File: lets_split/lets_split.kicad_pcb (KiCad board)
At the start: 2 copper layers, 112 x 79 mm, 62 parts, among them J1 3PIN, J2 6PIN, J3 3PIN, SW1 SW_PUSH, SW10 SW_PUSH, SW11 SW_PUSH, SW12 SW_PUSH, SW13 SW_PUSH, SW14 SW_PUSH, SW15 SW_PUSH, SW16 SW_PUSH, SW17 SW_PUSH, SW18 SW_PUSH, SW19 SW_PUSH, SW2 SW_PUSH, SW21 SW_PUSH, SW22 SW_PUSH, SW23 SW_PUSH, SW3 SW_PUSH, SW4 SW_PUSH, SW5 SW_PUSH, SW6 SW_PUSH, SW7 SW_PUSH, SW8 SW_PUSH, SW9 SW_PUSH, U2 HOLE, U3 HOLE, U4 HOLE, U5 HOLE

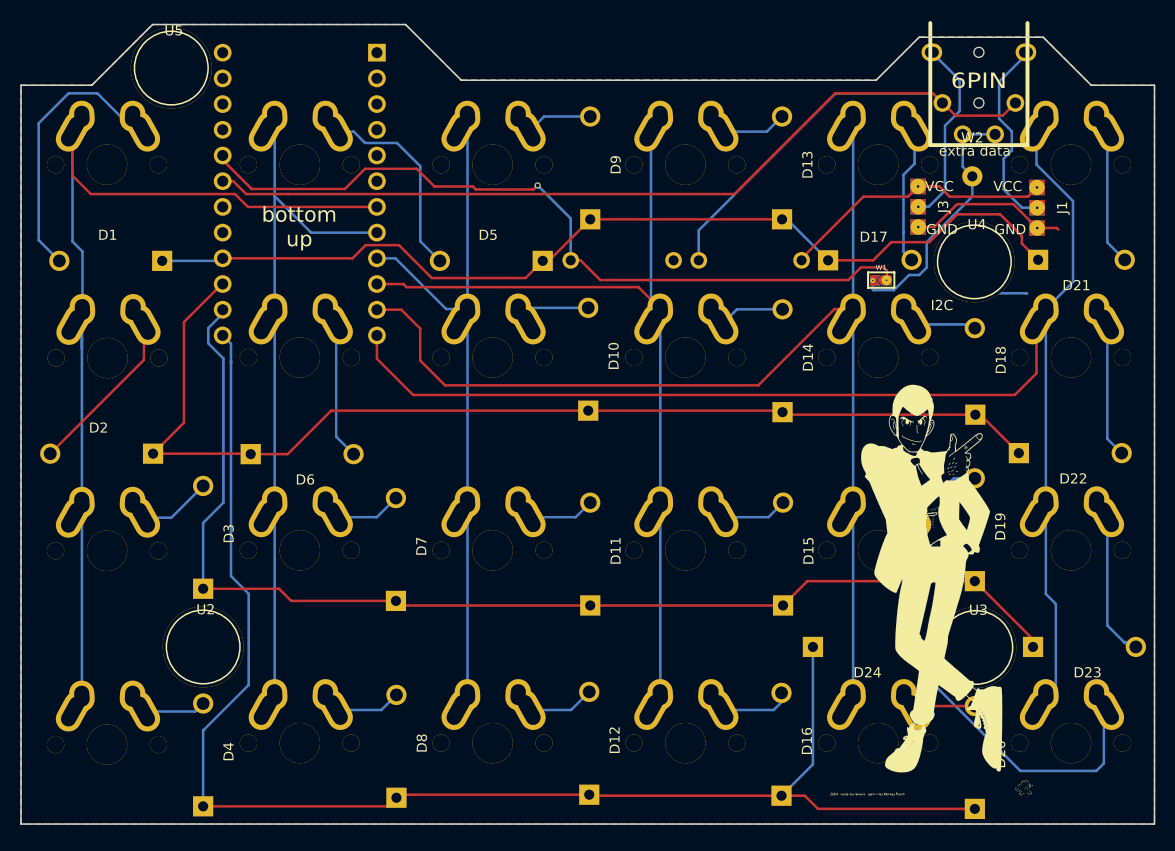
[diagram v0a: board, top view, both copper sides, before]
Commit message: Rev 1 complete
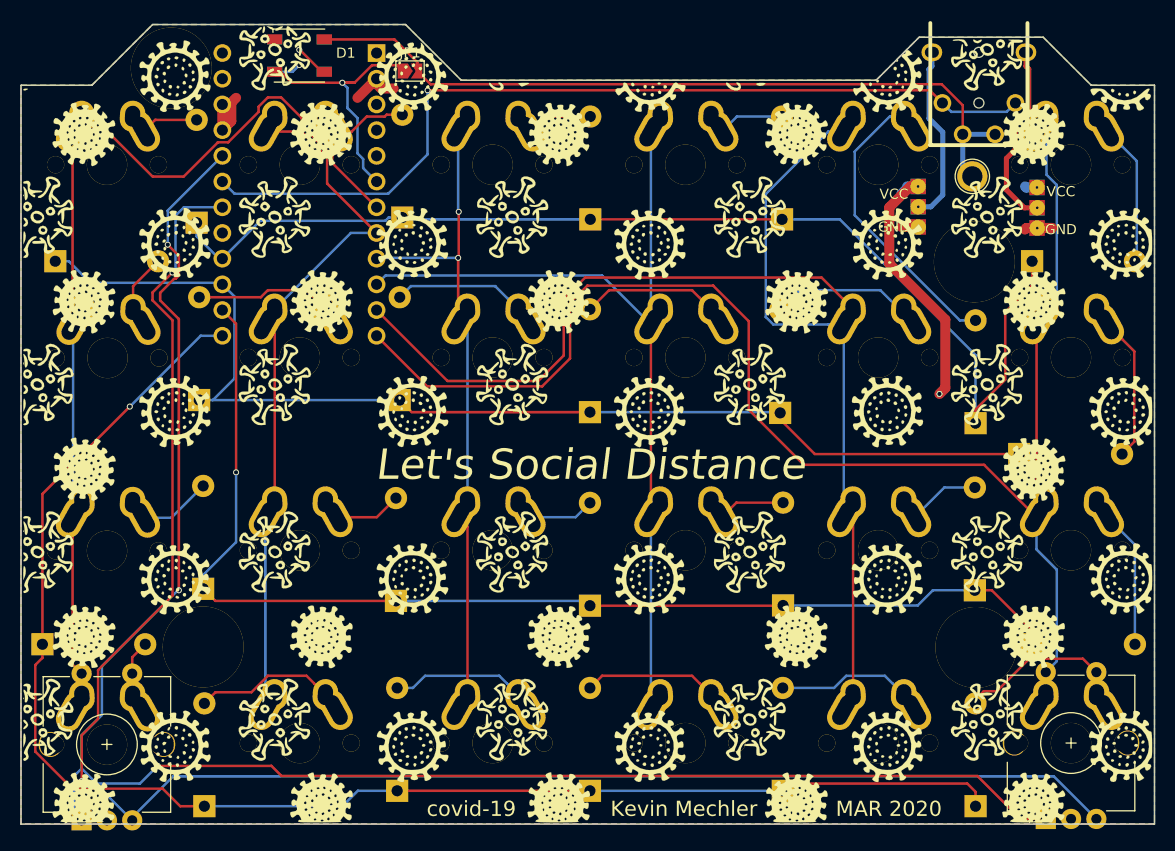
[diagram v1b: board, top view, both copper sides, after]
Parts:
- removed the D3 at (55.0, 88.8)
- removed the G*** at (118.8, 78.0)
- removed the G*** at (127.0, 87.8)
- removed R1, R2: R, footprint:RESISTOR
- removed the SW14 at (102.7, 65.9)
- removed the SW18 at (121.7, 65.9)
- removed the SW4 at (45.5, 104.2)
- removed U5: HOLE, prettylib:HOLE
- removed W2: TEST_1P, Wire_Pads:SolderWirePad_single_2mmDrill
- added D1: Inolux_IN-PI554FCH, LED_SMD:LED_Inolux_IN-PI554FCH_PLCC4_5.0x5.0mm_P3.2mm, F.Cu at (64.5, 36.1)
- added D25: D, LetsSplitSingle:D_DO-41_SOD81_P10.16mm_Horizontal, F.Cu at (136.9, 94.2)
- added D26: D, LetsSplitSingle:D_DO-41_SOD81_P10.16mm_Horizontal, F.Cu at (131.3, 110.2)
- added G***: LOGO, LSD_KB:coronaBack_with_space_for_text, B.Cu at (93.0, 72.5)
- added G***: LOGO, LSD_KB:coronaFront, F.Cu at (93.0, 72.5)
- added J4: 3PIN, LetsSplitSingle:3_pin_TP, F.Cu at (127.7, 51.0)
- added JP1: Jumper, Jumper:SolderJumper-2_P1.3mm_Open_TrianglePad1.0x1.5mm, F.Cu at (75.4, 37.6)
- added SW1: Rotary_Encoder_Switch, Rotary_Encoder:RotaryEncoder_Alps_EC12E-Switch_Vertical_H20mm, F.Cu at (43.0, 111.6)
- added SW15: SW_PUSH, flipalps:MXALPS_FLIP, F.Cu at (102.7, 65.9)
- added SW19: SW_PUSH, flipalps:MXALPS_FLIP, F.Cu at (121.7, 65.9)
- added SW24: SW_PUSH, flipalps:MXALPS_FLIP, F.Cu at (140.8, 65.9)
- added SW5: SW_PUSH, flipalps:MXALPS_FLIP, F.Cu at (45.5, 104.2)
- D10, D11, D12, D13, D14, D15, D16, D17, D18, D19, D20, D21, D22, D23, D24, D4, D5, D6, D7, D8, D9: footprint Diodes_ThroughHole:Diode_DO-41_SOD81_Horizontal_RM10 -> LetsSplitSingle:D_DO-41_SOD81_P10.16mm_Horizontal
- D2: value D -> Inolux_IN-PI554FCH; footprint Diodes_ThroughHole:Diode_DO-41_SOD81_Horizontal_RM10 -> LED_SMD:LED_Inolux_IN-PI554FCH_PLCC4_5.0x5.0mm_P3.2mm; moved to B.Cu
- D3: renamed from D1; footprint Diodes_ThroughHole:Diode_DO-41_SOD81_Horizontal_RM10 -> LetsSplitSingle:D_DO-41_SOD81_P10.16mm_Horizontal
- J1: value 3PIN -> Pro Micro 5V; footprint prettylib:jumper -> LetsSplitSingle:Pro_Micro; moved to B.Cu
- J2: value 6PIN -> 3PIN; footprint footprint:4pin35mmAudio -> LetsSplitSingle:3_pin_TP
- J3: value 3PIN -> 6PIN; footprint prettylib:jumper -> LetsSplitSingle:4pin35mmAudio
- SW22: value SW_PUSH -> Rotary_Encoder_Switch; footprint flipalps:MXALPS_FLIP -> Rotary_Encoder:RotaryEncoder_Alps_EC12E-Switch_Vertical_H20mm
- U1: value (none) -> HOLE; footprint footprint:TEENSY_2.0 -> LetsSplitSingle:LS_HOLE; moved to F.Cu
- U2, U3, U4: footprint prettylib:HOLE -> LetsSplitSingle:LS_HOLE
- W1: value TEST -> TEST_1P; footprint prettylib:JUMPER_SMD_2DUB -> TestPoint:TestPoint_Plated_Hole_D2.0mm
- moved U3 98.0 mm to (53.5, 38.0)
- moved U1 82.2 mm to (133.0, 95.2), turned to 0 degrees
- moved J1 74.9 mm to (64.5, 49.8), turned to 270 degrees
- moved D4 55.8 mm to (40.4, 56.4), turned to 0 degrees
- moved D10 54.5 mm to (55.1, 110.2)
- moved D14 53.4 mm to (74.2, 108.7)
- moved D18 53.2 mm to (93.2, 108.7)
- moved D5 46.6 mm to (55.0, 88.8), turned to 90 degrees
- moved SW22 45.7 mm to (138.3, 111.5), turned to 90 degrees
- moved D8 43.9 mm to (54.6, 70.1)
- moved D20 43.6 mm to (112.0, 71.4)
- moved D12 43.3 mm to (74.4, 70.1)
- moved D13 42.6 mm to (93.2, 90.4)
- moved D16 42.4 mm to (93.2, 71.3)
- moved D9 42.3 mm to (74.0, 90.0)
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- gave numbers to parts that had none: 2
- renumbered SW9 to SW10, SW10 to SW11, SW11 to SW12, SW12 to SW13, SW13 to SW14, SW15 to SW16, SW16 to SW17, SW17 to SW18, SW1 to SW2, SW19 to SW20, SW21 to SW23, SW23 to SW25, SW2 to SW3, SW3 to SW4, SW5 to SW6, SW6 to SW7, SW7 to SW8, SW8 to SW9
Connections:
- D10 pad 1: row1 -> row3
- D11 pad 1: row2 -> row0
- D12 pad 1: row3 -> row1
- D13 pad 1: row0 -> row2
- D14 pad 1: row1 -> row3
- D15 pad 1: row2 -> row0
- D16 pad 1: row3 -> row1
- D17 pad 1: row0 -> row2
- D18 pad 1: row1 -> row3
- D19 pad 1: row2 -> row0
- D2 pad 1: row1 -> GND
- D20 pad 1: row3 -> row1
- D21 pad 1: row0 -> row2
- D22 pad 1: row1 -> row3
- D23 pad 1: row2 -> row0
- D24 pad 1: row3 -> row1
- D4 pad 1: row3 -> row1
- D5 pad 1: row0 -> row2
- D6 pad 1: row1 -> row3
- D7 pad 1: row2 -> row0
- D8 pad 1: row3 -> row1
- D9 pad 1: row0 -> row2
- J1 pad 1: GND -> Net-(J1-Pad1)
- J1 pad 2: Net-(J1-Pad2) -> GND
- J1 pad 3: VCC -> Net-(J1-Pad3)
- J2 pad 1: Net-(J1-Pad2) -> GND
- J2 pad 2: data -> Net-(J2-Pad2)
- J2 pad 3: xtradata -> VCC
- J3 pad 1: GND -> Net-(J2-Pad2)
- J3 pad 2: Net-(J2-Pad4) -> data
- J3 pad 3: VCC -> xtradata
- SW10 pad 2: Net-(D9-Pad2) -> Net-(D11-Pad2)
- SW11 pad 2: Net-(D10-Pad2) -> Net-(D12-Pad2)
- SW12 pad 2: Net-(D11-Pad2) -> Net-(D13-Pad2)
- SW13 pad 2: Net-(D12-Pad2) -> Net-(D14-Pad2)
- SW14 pad 2: Net-(D13-Pad2) -> Net-(D15-Pad2)
- SW16 pad 2: Net-(D15-Pad2) -> Net-(D17-Pad2)
- SW17 pad 2: Net-(D16-Pad2) -> Net-(D18-Pad2)
- SW18 pad 2: Net-(D17-Pad2) -> Net-(D19-Pad2)
- SW20 pad 2: Net-(D19-Pad2) -> Net-(D21-Pad2)
- SW21 pad 2: Net-(D20-Pad2) -> Net-(D22-Pad2)
- SW23 pad 2: Net-(D21-Pad2) -> Net-(D23-Pad2)
- SW25 pad 2: Net-(D23-Pad2) -> Net-(D25-Pad2)
- SW26 pad 2: Net-(D24-Pad2) -> Net-(D26-Pad2)
- SW3 pad 2: Net-(D2-Pad2) -> Net-(D4-Pad2)
- SW4 pad 2: Net-(D3-Pad2) (its old number) -> Net-(D5-Pad2)
- SW6 pad 2: Net-(D5-Pad2) -> Net-(D7-Pad2)
- SW7 pad 2: Net-(D6-Pad2) -> Net-(D8-Pad2)
- SW8 pad 2: Net-(D7-Pad2) -> Net-(D9-Pad2)
- SW9 pad 2: Net-(D8-Pad2) -> Net-(D10-Pad2)
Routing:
- net EncA: track 0.00 -> 173.4 mm, vias 0 -> 3
- net EncB: track 0.00 -> 172.0 mm, vias 0 -> 2
- net Net-(R1-Pad2): track 77.0 -> 0.00 mm, vias 1 -> 0
- net xtradata: track 25.8 -> 76.9 mm
- net data: track 117.5 -> 88.0 mm, vias 0 -> 1
- net Net-(D1-Pad2): track 0.00 -> 26.4 mm, vias 0 -> 1
- net Net-(D3-Pad2): track 27.6 -> 5.74 mm
- net Net-(D19-Pad2): track 7.54 -> 28.8 mm
- net Net-(J1-Pad2): track 19.5 -> 0.00 mm
- net Net-(J2-Pad4): track 18.7 -> 0.00 mm
- net Net-(J2-Pad2): track 0.00 -> 18.4 mm
- net Net-(J3-Pad4): track 0.00 -> 17.7 mm
- net Net-(D26-Pad2): track 0.00 -> 16.8 mm
- net Net-(D2-Pad2): track 16.6 -> 0.00 mm
- net Net-(D24-Pad2): track 30.5 -> 14.4 mm
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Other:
- board text added: "Kevin Mechler"
- board text added: "Let's Social Distance"
- board text added: "MAR 2020"
- board text added: "Original By Wootpatoot"
- board text added: "covid-19"
- board text removed: "By Wootpatoot"
- board text removed: "I2C"
- board text removed: "LET'S SPLIT"
- board text removed: "bottom up"
- board text removed: "extra data"
- board text removed: "top up"
